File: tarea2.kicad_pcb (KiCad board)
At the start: 2 copper layers, 13 parts, among them IC1 LDO40LPURY, J1 Conn_01x02_Pin, J2 Conn_01x06_Pin, U1 STM32G030K8Tx

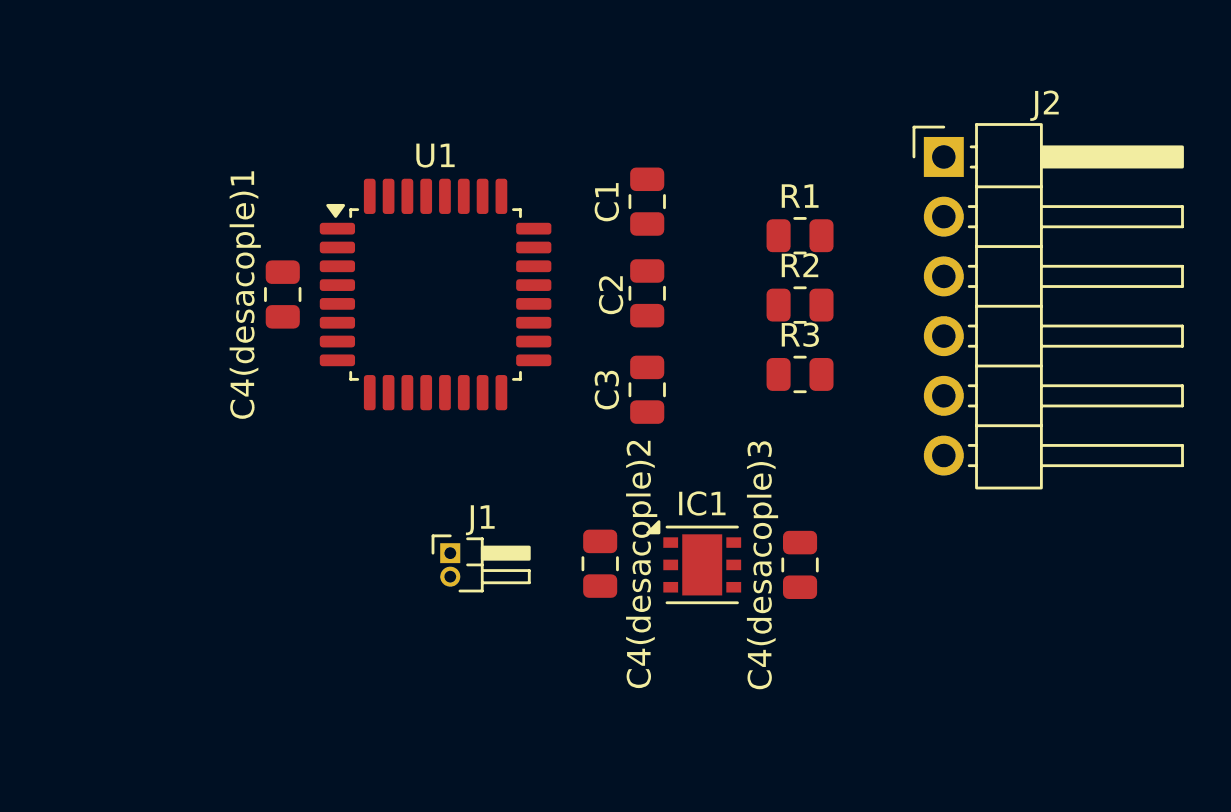
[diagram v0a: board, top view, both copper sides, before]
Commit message: Colocación inicial de los elementos en la PCB
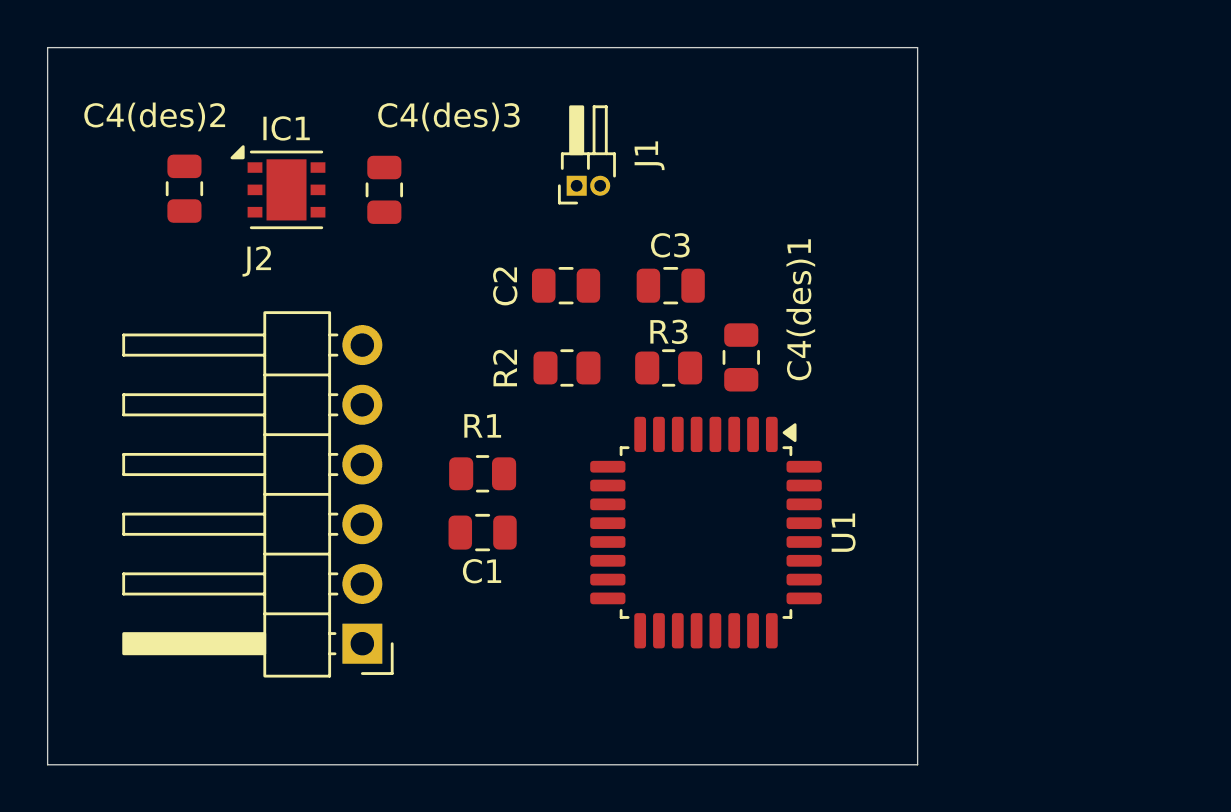
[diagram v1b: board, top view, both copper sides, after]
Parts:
- moved J2 32.3 mm to (146.9, 123.8), turned to 180 degrees
- moved C4(des)2 23.8 mm to (139.3, 104.5), turned to 90 degrees
- moved C4(des)3 23.8 mm to (147.8, 104.5)
- moved IC1 23.8 mm to (143.7, 104.5)
- moved C4(des)1 19.7 mm to (163.0, 111.7)
- moved R1 16.9 mm to (152.0, 116.6), turned to 180 degrees
- moved J1 16.5 mm to (156.0, 104.4), turned to 90 degrees
- moved C1 15.7 mm to (152.0, 119.1), turned to 180 degrees
- moved U1 15.3 mm to (161.5, 119.1), turned to -90 degrees
- moved R2 10.3 mm to (155.6, 112.1), turned to 180 degrees
- moved R3 5.59 mm to (159.9, 112.1)
- moved C3 4.54 mm to (160.0, 108.6), turned to 0 degrees
- moved C2 3.47 mm to (155.6, 108.6), turned to 180 degrees
- renumbered C4(desacople)1 to C4(des)1, C4(desacople)2 to C4(des)2, C4(desacople)3 to C4(des)3
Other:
- board outline added: 37 x 30.5 mm
